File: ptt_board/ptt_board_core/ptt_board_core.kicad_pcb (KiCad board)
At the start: 2 copper layers, 25 x 25 mm, 14 parts, among them P0.03 TestPoint, P0.07 TestPoint, P0.30 TestPoint, P26 Conn_01x01_Pin, U1 SKB369

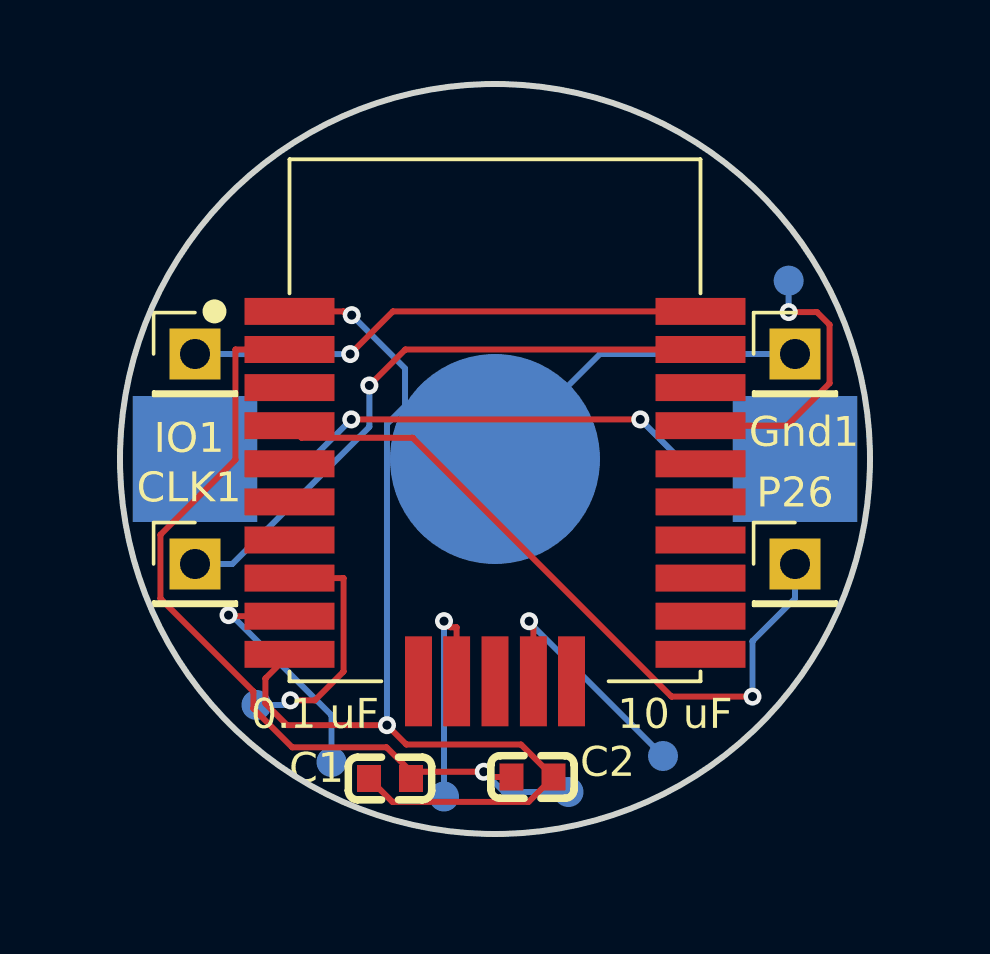
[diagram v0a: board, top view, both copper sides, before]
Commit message: [WIP] Started net rev of ptt board and radio board
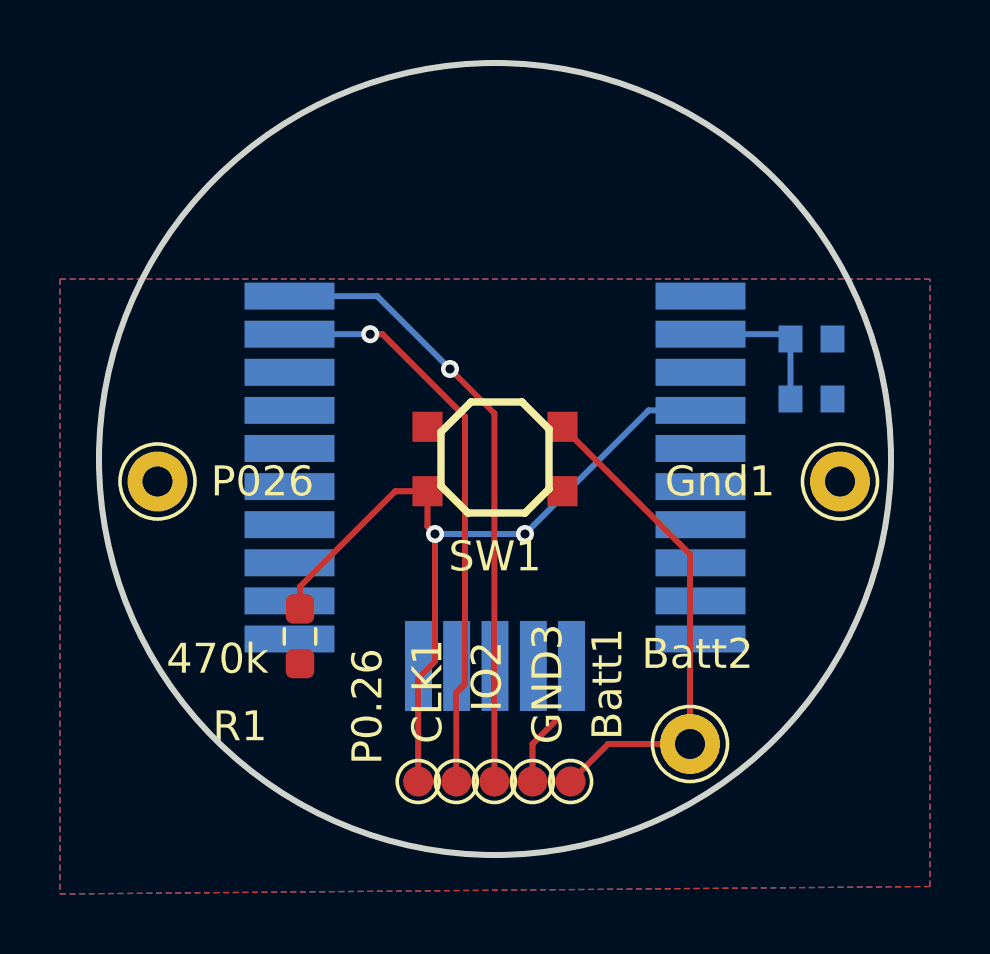
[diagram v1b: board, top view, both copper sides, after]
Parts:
- removed BT1: MY-1632-03-R, Project_components:BAT-SMD_MY-1632-03
- removed Batt+1, P.0.31, P0.03, P0.07, P0.30, Reset1: TestPoint, TestPoint:TestPoint_Pad_D1.0mm
- removed IO1, P26: Conn_01x01_Pin, Connector_PinHeader_2.54mm:PinHeader_1x01_P2.54mm_Vertical
- added Batt1: TestPoint, TestPoint:TestPoint_Pad_D1.0mm, F.Cu at (102.5, 110.8)
- added Batt2: Conn_01x01_Pin, Connector_Pin:Pin_D1.0mm_L10.0mm, F.Cu at (106.5, 109.5)
- added GND3: TestPoint, TestPoint:TestPoint_Pad_D1.0mm, F.Cu at (101.2, 110.8)
- added IO2: TestPoint, TestPoint:TestPoint_Pad_D1.0mm, F.Cu at (100.0, 110.8)
- added P0.26: TestPoint, TestPoint:TestPoint_Pad_D1.0mm, F.Cu at (97.4, 110.8)
- added P026: Conn_01x01_Pin, Connector_Pin:Pin_D1.0mm_L10.0mm, F.Cu at (88.8, 100.8)
- added R1: 470k, Resistor_SMD:R_0603_1608Metric_Pad0.98x0.95mm_HandSolder, F.Cu at (93.5, 105.9)
- added SW1: RKB2SJG250SMTRLFS, Project_components:Push button C2927788, F.Cu at (100.0, 100.0)
- C1, C2, U1: moved to B.Cu
- CLK1: value Conn_01x01_Pin -> TestPoint; footprint Connector_PinHeader_2.54mm:PinHeader_1x01_P2.54mm_Vertical -> TestPoint:TestPoint_Pad_D1.0mm
- Gnd1: footprint Connector_PinHeader_2.54mm:PinHeader_1x01_P2.54mm_Vertical -> Connector_Pin:Pin_D1.0mm_L10.0mm
- moved C1 20.3 mm to (110.5, 96.0), turned to 0 degrees
- moved C2 15.7 mm to (110.5, 98.0)
- moved CLK1 11.3 mm to (98.7, 110.8), turned to -90 degrees
- moved Gnd1 4.51 mm to (111.5, 100.8)
- moved U1 0.51 mm to (100.0, 98.2), turned to 180 degrees
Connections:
- U1 pad 12: Net-(U1-P0.03) -> unconnected-(U1-P0.03-Pad12)
- U1 pad 14: Net-(U1-P0.07) -> unconnected-(U1-P0.07-Pad14)
- U1 pad 22: Reset -> unconnected-(U1-P0.21/~{RESET}-Pad22)
- U1 pad 4: Net-(P26-Pin_1) -> P0.26
- U1 pad 6: unconnected-(U1-P0.28-Pad6) -> P0.28
- U1 pad 8: Net-(U1-P0.30) -> unconnected-(U1-P0.30-Pad8)
- U1 pad 9: Net-(U1-P0.31) -> unconnected-(U1-P0.31-Pad9)
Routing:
- net GND: track 51.4 -> 2.31 mm, vias 2 -> 0
- net P0.26: track 0.00 -> 27.2 mm, vias 0 -> 2
- net Net-(P26-Pin_1): track 24.2 -> 0.00 mm, vias 1 -> 0
- net unconnected-(BT1-Pad1): track 21.1 -> 0.00 mm, vias 2 -> 0
- net Reset: track 9.42 -> 0.00 mm, vias 1 -> 0
- net Net-(U1-P0.31): track 8.42 -> 0.00 mm, vias 1 -> 0
- net Net-(U1-P0.07): track 8.40 -> 0.00 mm, vias 1 -> 0
- net Net-(U1-P0.30): track 8.28 -> 0.00 mm, vias 1 -> 0
- net Net-(U1-P0.03): track 8.15 -> 0.00 mm, vias 1 -> 0
- net +BATT: track 29.0 -> 21.9 mm, vias 1 -> 0
- net SWDIO: track 17.4 -> 20.7 mm
- net SWDCLK: track 20.6 -> 19.3 mm
- added copper zone on B.Cu, net GND
- added copper zone on F.Cu, net GND
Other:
- board size 25 x 25 mm -> 26.4 x 26.4 mm
